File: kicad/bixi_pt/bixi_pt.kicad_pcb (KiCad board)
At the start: 2 copper layers, 47 x 21.6 mm, 9 parts, among them J1 Screw_Terminal_1x02, J2 CONN_01X03, J3 CONN_01X03

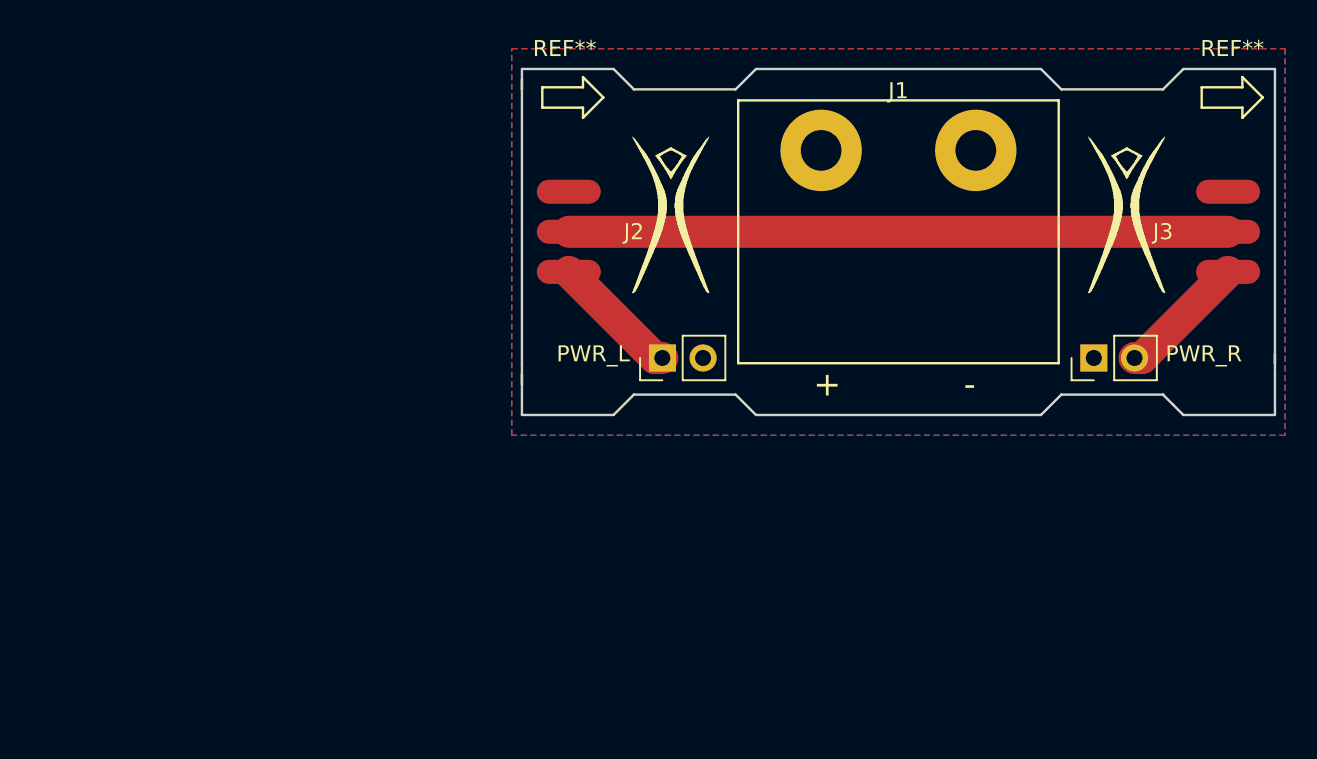
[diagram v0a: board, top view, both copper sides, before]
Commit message: new power injection board is ready
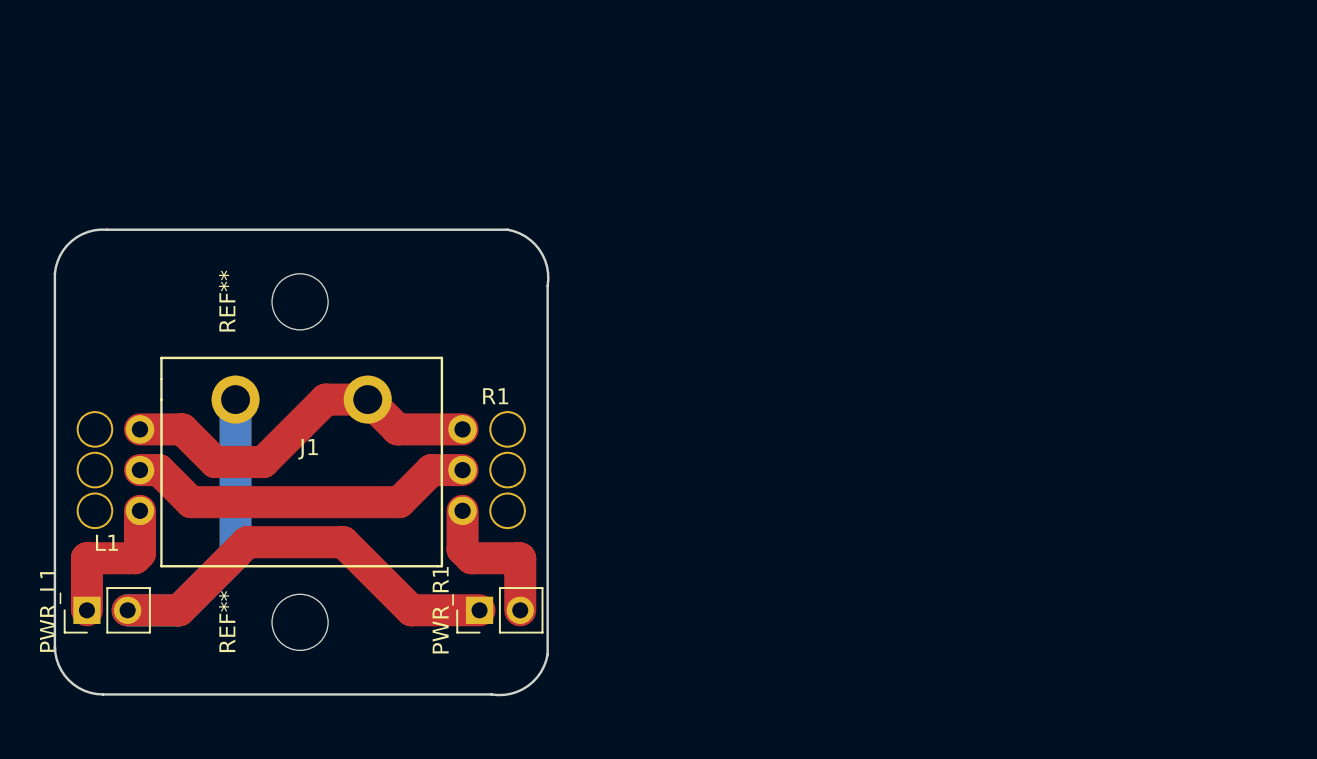
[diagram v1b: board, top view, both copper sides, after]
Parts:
- removed J2, J3: CONN_01X03, custom:PAD_3X_OVAL_WS2812B
- removed PWR_L, PWR_R: Jumper, Pin_Headers:Pin_Header_Straight_1x02_Pitch2.54mm
- removed the REF** at (188.5, 79.2)
- removed the REF** at (147.3, 79.2)
- removed burner-logo1, burner-logo2: , logos:burner-logo-fs
- added L1: CONN_01X03, custom:3-wire-hole-with-relief, F.Cu at (118.5, 102.5)
- added PWR_L1: Jumper, Pin_Headers:Pin_Header_Straight_1x02_Pitch2.54mm, F.Cu at (117.0, 111.2)
- added PWR_R1: Jumper, Pin_Headers:Pin_Header_Straight_1x02_Pitch2.54mm, F.Cu at (141.5, 111.2)
- added R1: CONN_01X03, custom:3-wire-hole-with-relief, F.Cu at (142.2, 102.5)
- added REF**: MountingHole_3.5mm, Mounting_Holes:MountingHole_3.5mm, F.Cu at (130.3, 92.0)
- added REF**: MountingHole_3.5mm, Mounting_Holes:MountingHole_3.5mm, F.Cu at (130.3, 112.0)
- J1: footprint custom:HP_9500_Terminal_Connector -> custom:OSTYK42102030-2P-Terminal
- moved J1 38.7 mm to (130.4, 98.1)
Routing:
- net /VCC: track 0.00 -> 43.3 mm
- net /GND: track 0.00 -> 23.4 mm
- net /DATA: track 41.1 -> 21.8 mm
- net /VCCR: track 8.06 -> 9.46 mm
- net /VCCL: track 8.06 -> 9.34 mm
- removed copper zone on F.Cu, net /GND
- removed copper zone on B.Cu, net /VCC
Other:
- board size 47 x 21.6 mm -> 30.8 x 29 mm
- board text removed: "+"
- board text removed: "-"

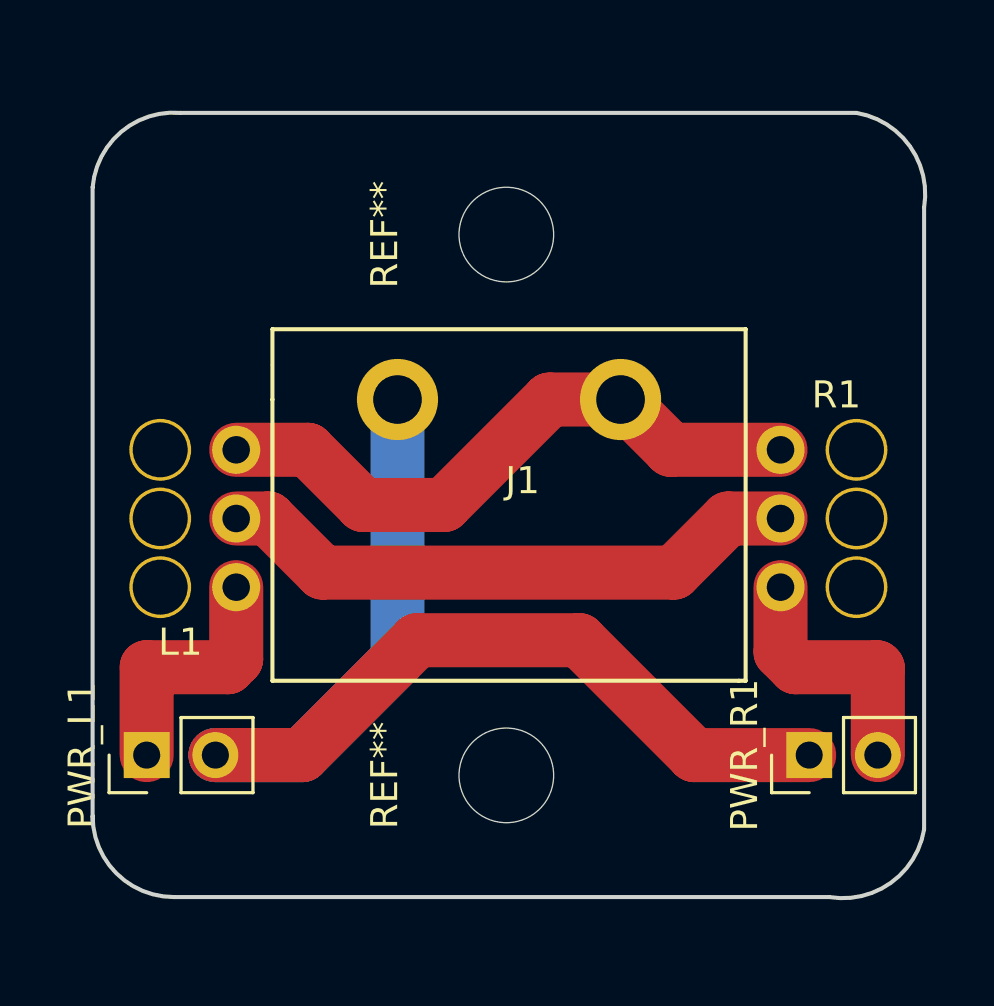
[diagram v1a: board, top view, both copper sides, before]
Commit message: fixes to boards, node still in progress
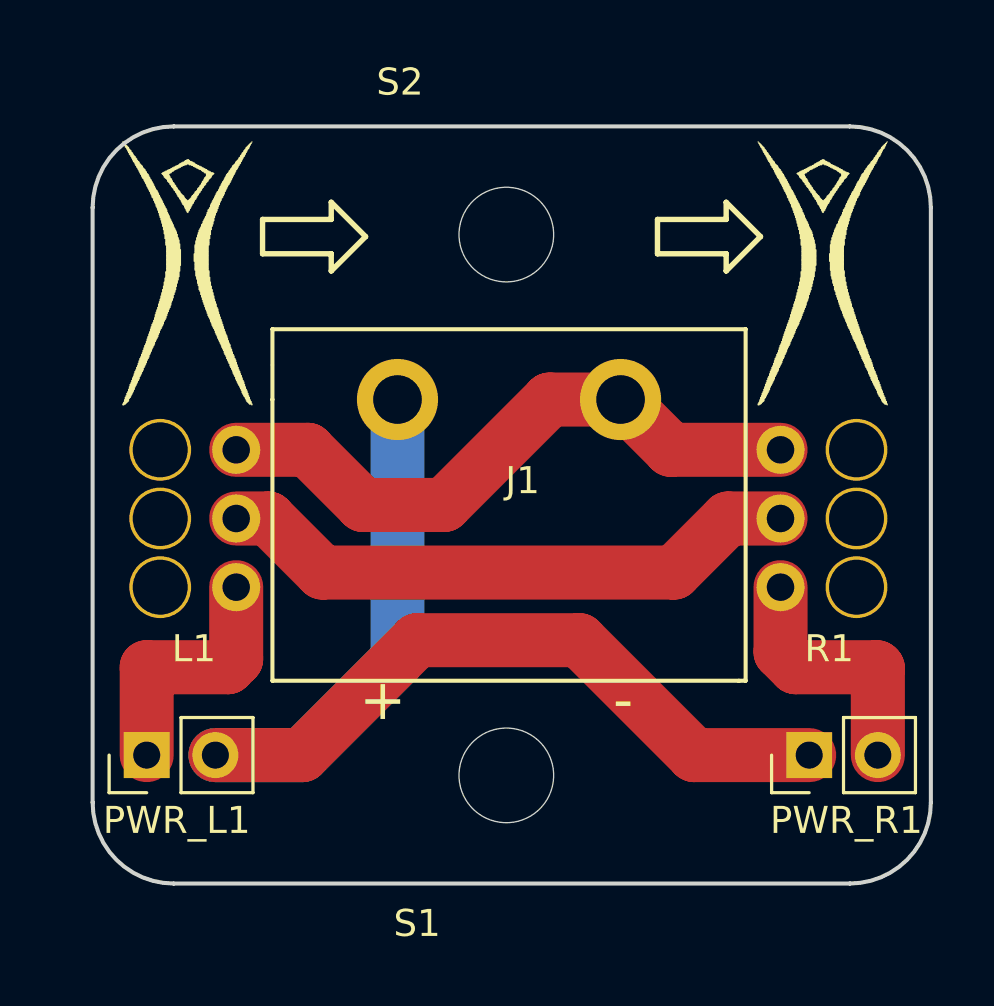
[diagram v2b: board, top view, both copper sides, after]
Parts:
- added burner-logo: , logos:burner-logo-fs, F.Cu at (114.9, 87.6)
- added burner-logo: , logos:burner-logo-fs, F.Cu at (138.4, 87.6)
- renumbered REF** to S1, REF** to S2
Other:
- board size 30.8 x 29 mm -> 31 x 28 mm
- board text added: "+"
- board text added: "-"
